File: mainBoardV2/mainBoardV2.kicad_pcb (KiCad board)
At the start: 2 copper layers, 41.7 x 49.6 mm, 24 parts, among them J1 USB4125-GF-A_REVA2, U3 MCP73871-2AAI_ML, U4 MPU6050_Module, U5 TPS61023DRLT

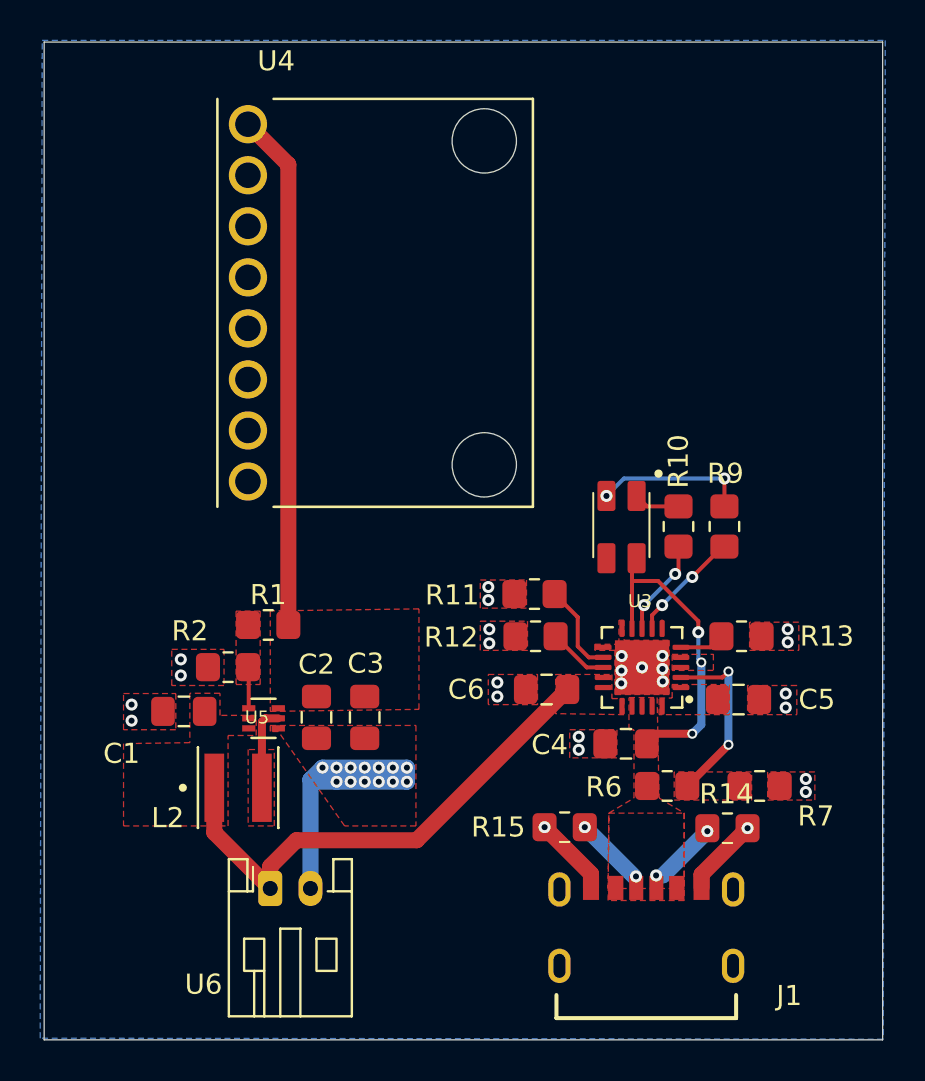
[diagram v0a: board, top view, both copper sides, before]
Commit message: 3.12.26.C1
Seems this board is close to done. Need to discuss where our pushbutton and on/of switch would connect.
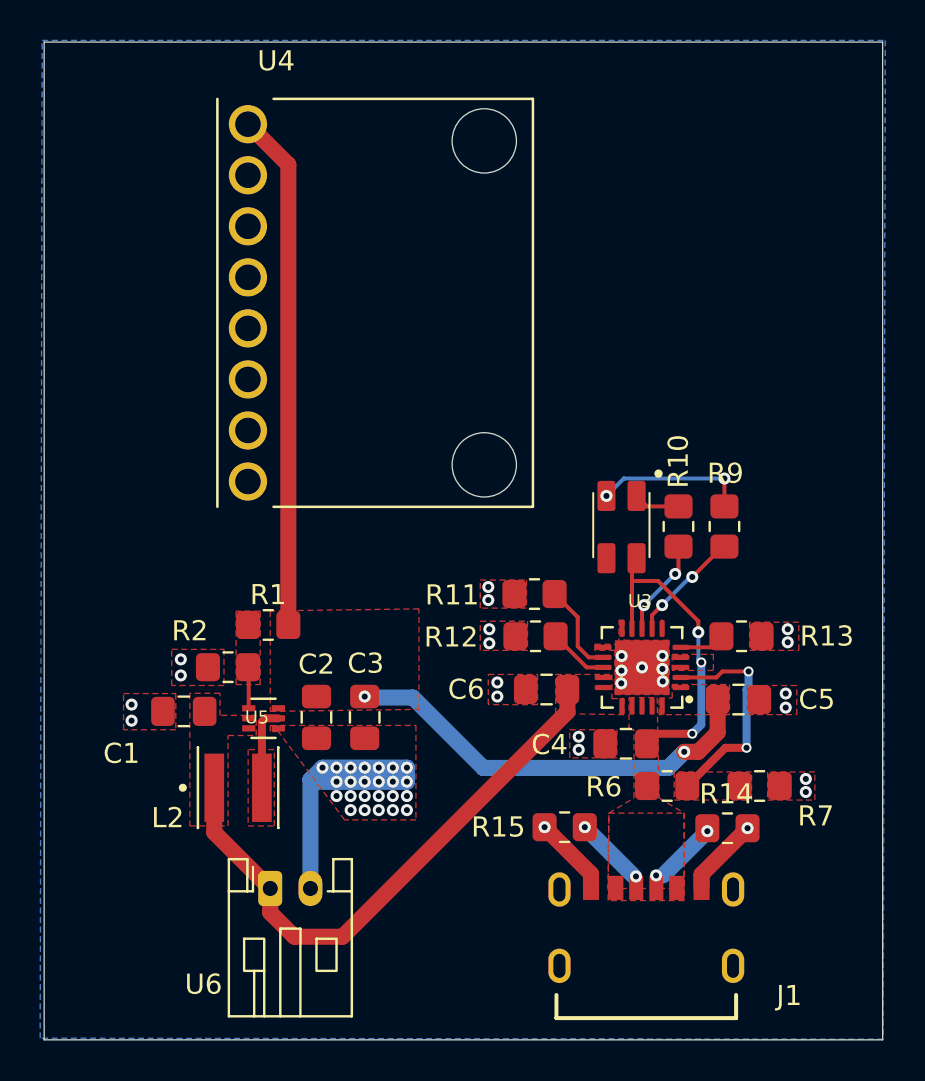
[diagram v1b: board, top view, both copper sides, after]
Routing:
- net /VoutBoost: track 25.8 -> 47.2 mm, vias 0 -> 2
- net /VBatt+: track 25.7 -> 28.4 mm
- net /VPCC: track 9.04 -> 11.1 mm
- net GND: track 24.6 -> 23.9 mm, vias 40 -> 51
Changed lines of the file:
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@@
-	)
-	(segment
-		(start 123.9475 116.324)
-		(end 124.418 115.8535)
-		(width 0.2)
-		(layer "F.Cu")
-		(net 4)
 	)
 	(segment
@@
 	)
 	(via
+		(at 106.4 121.2)
+		(size 0.6)
+		(drill 0.3)
+		(layers "F.Cu" "B.Cu")
+		(free yes)
+		(net 4)
+	)
+	(via
+		(at 105.7 121.2)
+		(size 0.6)
+		(drill 0.3)
+		(layers "F.Cu" "B.Cu")
+		(free yes)
+		(net 4)
+	)
+	(via
 		(at 102.2 119.7875)
 		(size 0.6)
@@
 	)
 	(via
+		(at 105 121.2)
+		(size 0.6)
+		(drill 0.3)
+		(layers "F.Cu" "B.Cu")
+		(free yes)
+		(net 4)
+	)
+	(via
 		(at 125.35 113.55)
 		(size 0.6)
@@
 	)
 	(via
+		(at 103.6 121.2)
+		(size 0.6)
+		(drill 0.3)
+		(layers "F.Cu" "B.Cu")
+		(free yes)
+		(net 4)
+	)
+	(via
 		(at 95.15 114.4)
 		(size 0.6)
@@
 	)
 	(via
+		(at 104.3 121.2)
+		(size 0.6)
+		(drill 0.3)
+		(layers "F.Cu" "B.Cu")
+		(free yes)
+		(net 4)
+	)
+	(via
+		(at 103.6 121.9)
+		(size 0.6)
+		(drill 0.3)
+		(layers "F.Cu" "B.Cu")
+		(free yes)
+		(net 4)
+	)
+	(via
 		(at 104.3 120.4875)
 		(size 0.6)
@@
 	)
 	(via
+		(at 105.7 121.9)
+		(size 0.6)
+		(drill 0.3)
+		(layers "F.Cu" "B.Cu")
+		(free yes)
+		(net 4)
+	)
+	(via
+		(at 105 121.9)
+		(size 0.6)
+		(drill 0.3)
+		(layers "F.Cu" "B.Cu")
+		(free yes)
+		(net 4)
+	)
+	(via
 		(at 113.25 122.75)
 		(size 0.6)
@@
 	)
 	(via
+		(at 102.9 121.2)
+		(size 0.6)
+		(drill 0.3)
+		(layers "F.Cu" "B.Cu")
+		(free yes)
+		(net 4)
+	)
+	(via
 		(at 125.25 116.8)
 		(size 0.6)
@@
 	)
 	(via
+		(at 104.3 121.9)
+		(size 0.6)
+		(drill 0.3)
+		(layers "F.Cu" "B.Cu")
+		(free yes)
+		(net 4)
+	)
+	(via
 		(at 118.1 114.8)
 		(size 0.6)
@@
 	(via
 		(at 114.95 118.9)
+		(size 0.6)
+		(drill 0.3)
+		(layers "F.Cu" "B.Cu")
+		(free yes)
+		(net 4)
+	)
+	(via
+		(at 106.4 121.9)
 		(size 0.6)
 		(drill 0.3)
@@
 	)
 	(segment
+		(start 123.4 115)
+		(end 122.1 115)
+		(width 0.2)
+		(layer "F.Cu")
+		(net 10)
+	)
+	(segment
+		(start 122.1 115)
+		(end 121.8 115.3)
+		(width 0.2)
+		(layer "F.Cu")
+		(net 10)
+	)
+	(segment
 		(start 120.35 120.7)
-		(end 122.4 118.65)
+		(end 122.25 118.8)
 		(width 0.4)
 		(layer "F.Cu")
@@
 	)
 	(segment
-		(start 120.035 115.3)
-		(end 122.1 115.3)
+		(start 121.8 115.3)
+		(end 120.035 115.3)
 		(width 0.2)
 		(layer "F.Cu")
@@
 	)
 	(segment
-		(start 122.1 115.3)
-		(end 122.4 115)
-		(width 0.2)
+		(start 122.25 118.8)
+		(end 123.3 118.8)
+		(width 0.4)
 		(layer "F.Cu")
 		(net 10)
 	)
 	(via
-		(at 122.4 118.65)
+		(at 123.3 118.8)
 		(size 0.5)
 		(drill 0.3)
@@
 	)
 	(via
-		(at 122.4 115)
+		(at 123.4 115)
 		(size 0.5)
 		(drill 0.3)
@@
 	)
 	(segment
-		(start 122.4 118.65)
-		(end 122.4 115)
+		(start 123.3 115.9)
+		(end 123.3 118.8)
+		(width 0.4)
+		(layer "B.Cu")
+		(net 10)
+	)
+	(segment
+		(start 123.4 115.8)
+		(end 123.3 115.9)
+		(width 0.4)
+		(layer "B.Cu")
+		(net 10)
+	)
+	(segment
+		(start 123.4 115)
+		(end 123.4 115.8)
 		(width 0.4)
 		(layer "B.Cu")
@@
 	)
 	(segment
-		(start 106.8875 123.4)
+		(start 100.8 128.2)
+		(end 103.2 128.2)
+		(width 0.8)
+		(layer "F.Cu")
+		(net 16)
+	)
+	(segment
+		(start 99.6 127)
+		(end 100.8 128.2)
+		(width 0.8)
+		(layer "F.Cu")
+		(net 16)
+	)
+	(segment
+		(start 114.3875 117.0125)
 		(end 114.3875 115.9)
-		(width 0.8)
-		(layer "F.Cu")
-		(net 16)
-	)
-	(segment
-		(start 99.6 125.8)
-		(end 99.6 124.7)
 		(width 0.8)
 		(layer "F.Cu")
@@
 	)
 	(segment
-		(start 99.6 124.7)
-		(end 100.9 123.4)
+		(start 99.6 125.8)
+		(end 99.6 127)
 		(width 0.8)
 		(layer "F.Cu")
@@
 	)
 	(segment
-		(start 100.9 123.4)
-		(end 106.8875 123.4)
+		(start 103.2 128.2)
+		(end 114.3875 117.0125)
 		(width 0.8)
 		(layer "F.Cu")
@@
 	)
 	(segment
-		(start 121.8565 115.8)
-		(end 121.8725 115.816)
-		(width 0.2)
+		(start 121.8625 116.4)
+		(end 121.8625 118.040996)
+		(width 0.8)
+		(layer "F.Cu")
+		(net 17)
+	)
+	(segment
+		(start 121.8625 118.040996)
+		(end 120.903496 119)
+		(width 0.8)
 		(layer "F.Cu")
 		(net 17)
@@
 	)
 	(segment
+		(start 120.903496 119)
+		(end 120.2 119)
+		(width 0.8)
+		(layer "F.Cu")
+		(net 17)
+	)
+	(segment
 		(start 100.5 89.78)
 		(end 98.49 87.77)
 		(width 0.8)
 		(layer "F.Cu")
+		(net 17)
+	)
+	(via
+		(at 120.2 119)
+		(size 0.6)
+		(drill 0.3)
+		(layers "F.Cu" "B.Cu")
+		(net 17)
+	)
+	(via
+		(at 104.3 116.25)
+		(size 0.6)
+		(drill 0.3)
+		(layers "F.Cu" "B.Cu")
+		(net 17)
+	)
+	(segment
+		(start 104.35 116.3)
+		(end 104.3 116.25)
+		(width 0.8)
+		(layer "B.Cu")
+		(net 17)
+	)
+	(segment
+		(start 110.201 119.801)
+		(end 106.7 116.3)
+		(width 0.8)
+		(layer "B.Cu")
+		(net 17)
+	)
+	(segment
+		(start 120.2 119)
+		(end 119.399 119.801)
+		(width 0.8)
+		(layer "B.Cu")
+		(net 17)
+	)
+	(segment
+		(start 119.399 119.801)
+		(end 110.201 119.801)
+		(width 0.8)
+		(layer "B.Cu")
+		(net 17)
+	)
+	(segment
+		(start 106.7 116.3)
+		(end 104.35 116.3)
+		(width 0.8)
+		(layer "B.Cu")
 		(net 17)
 	)
@@
 		(polygon
 			(pts
-				(xy 106.85 117.6875) (xy 106.85 122.6875) (xy 103.3 122.6875) (xy 100 117.9875) (xy 99.6 117.9875)
+				(xy 106.85 117.6875) (xy 106.85 122.3875) (xy 103.3 122.3875) (xy 100 117.9875) (xy 99.6 117.9875)
 				(xy 99.6 117.6875)
 			)
@@
 			(pts
 				(xy 97.5 122.6875) (xy 97.5 118.1875) (xy 98.9 118.1875) (xy 98.9 117.1875) (xy 97.1 117.1875) (xy 97.1 116.0875)
-				(xy 95.6 116.0875) (xy 95.6 118.54375) (xy 92.3 118.59375) (xy 92.3 122.6875)
+				(xy 95.6 116.0875) (xy 95.6 118.54375) (xy 95.6 118.59375) (xy 95.6 122.6875)
 			)
 		)
